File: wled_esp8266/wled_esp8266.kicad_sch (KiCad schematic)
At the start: 34 parts, among them J1 PWR, J2 Conn_01x05, J3 Screw_Terminal_01x04, J4 LED_STRIPT, J5 USB_B_Micro, Q1 IRF3708, Q2 IRF3708, Q3 IRF3708, U1 ESP-12F, U2 AMS1117-3.3

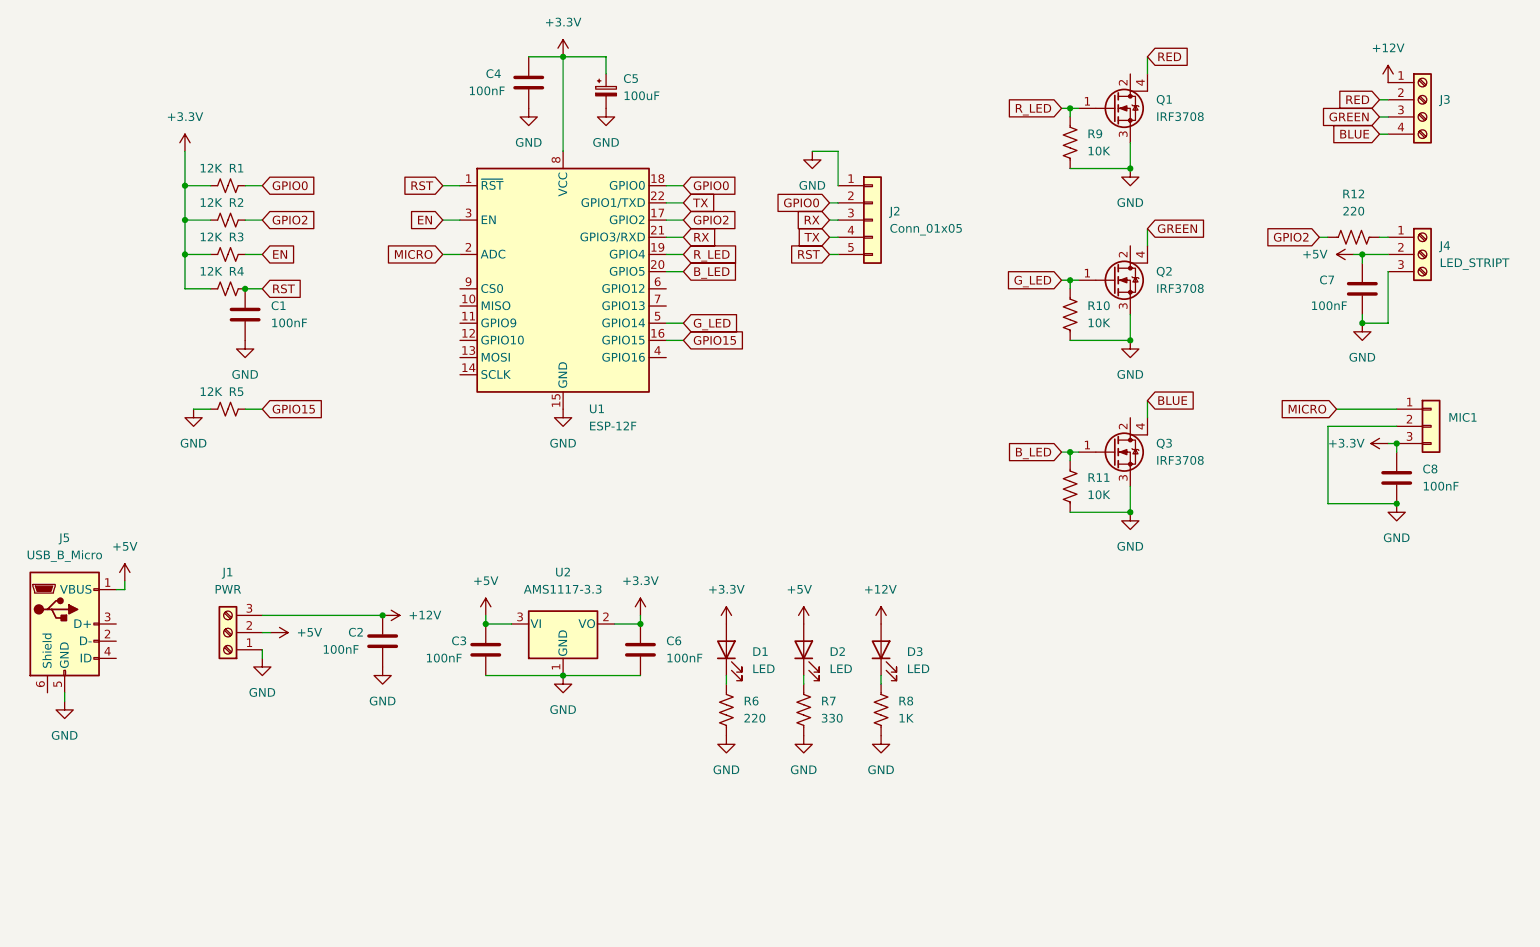
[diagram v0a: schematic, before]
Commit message: update new pcb
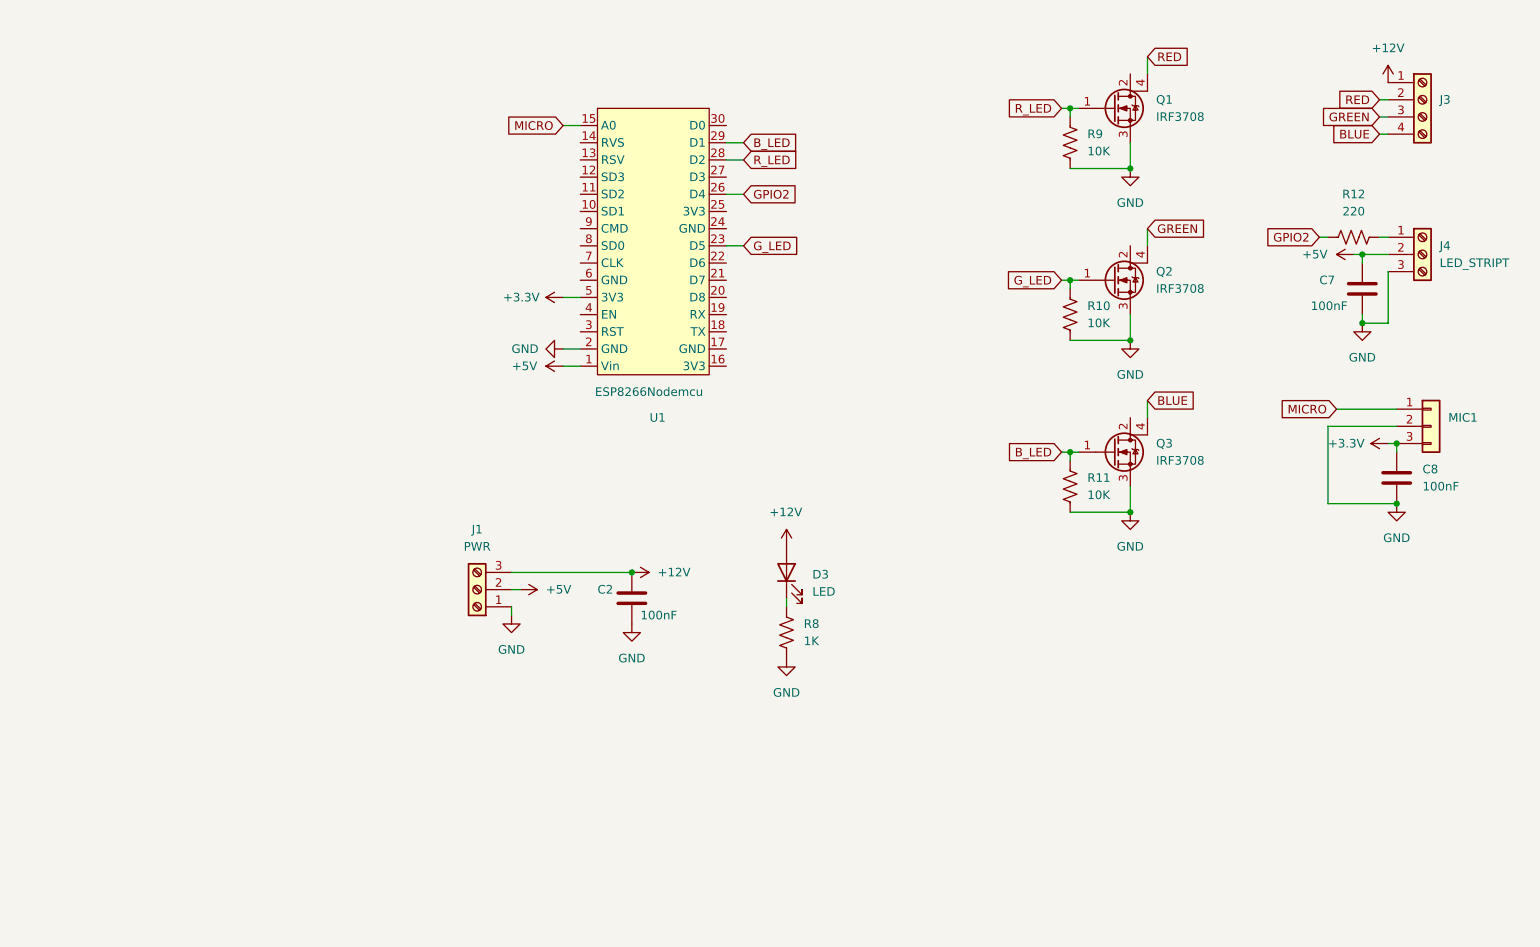
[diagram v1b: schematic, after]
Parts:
- removed C1, C3, C4, C6: 100nF, Capacitor_SMD:C_0805_2012Metric_Pad1.18x1.45mm_HandSolder, symbol Device:C
- removed C5: 100uF, Capacitor_Tantalum_SMD:CP_EIA-3528-12_Kemet-T_Pad1.50x2.35mm_HandSolder, symbol Device:C_Polarized_Small
- removed D1, D2: LED, LED_SMD:LED_0805_2012Metric_Pad1.15x1.40mm_HandSolder, symbol Device:LED
- removed J2: Conn_01x05, Connector_PinSocket_2.54mm:PinSocket_1x05_P2.54mm_Vertical, symbol Connector_Generic:Conn_01x05
- removed J5: USB_B_Micro, Connector_USB:USB_Micro, symbol Connector:USB_B_Micro
- removed R1, R2, R3, R4, R5: 12K, Resistor_SMD:R_0805_2012Metric_Pad1.20x1.40mm_HandSolder, symbol Device:R_Small_US
- removed R6: 220, Resistor_SMD:R_0805_2012Metric_Pad1.20x1.40mm_HandSolder, symbol Device:R_US
- removed R7: 330, Resistor_SMD:R_0805_2012Metric_Pad1.20x1.40mm_HandSolder, symbol Device:R_US
- removed U1: ESP-12F, RF_Module:ESP-12E, symbol RF_Module:ESP-12F
- removed U2: AMS1117-3.3, Package_TO_SOT_SMD:SOT-223-3_TabPin2, symbol Regulator_Linear:AMS1117-3.3
- added U1: ESP8266Nodemcu, Module:ESP8266Nodemcu, symbol MCU_Module:ESP8266Nodemcu
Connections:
- net +3V3: now also U1.5 (3V3)
- net +5V: now also U1.1 (Vin)
- net B_LED: now also U1.29 (D1)
- net GND: now also U1.2 (GND)
- net GPIO2: now also U1.26 (D4)
- net G_LED: now also U1.23 (D5)
- net MICRO: now also U1.15 (A0)
- net R_LED: now also U1.28 (D2)
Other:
- moved on the sheet: C2, D3, R8

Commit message: update PCB
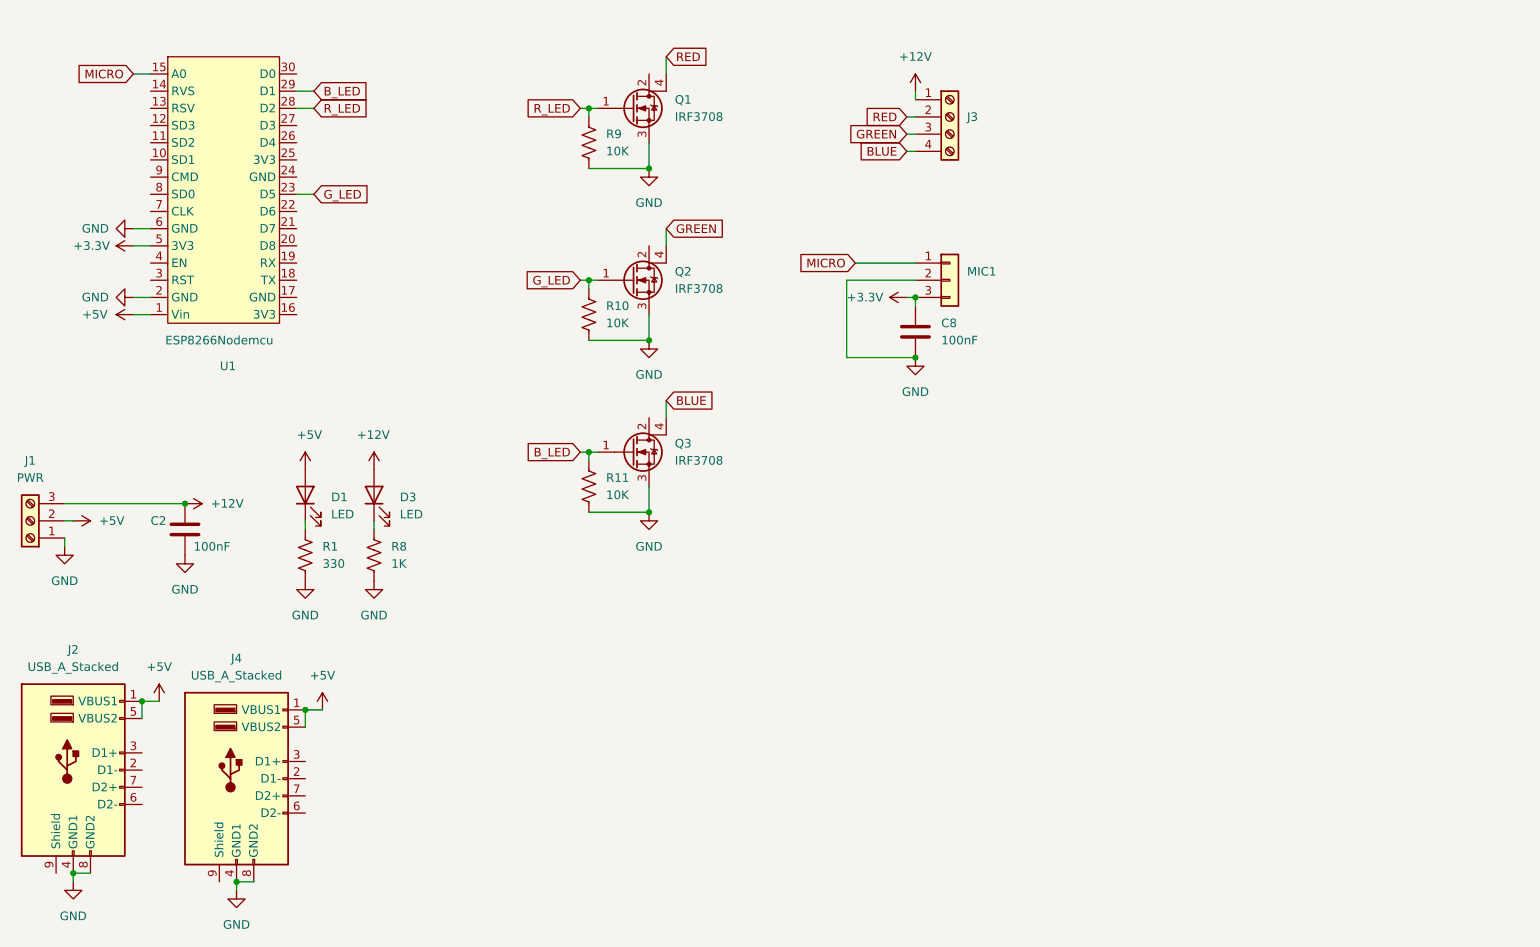
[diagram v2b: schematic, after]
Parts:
- removed C7: 100nF, Capacitor_SMD:C_0805_2012Metric_Pad1.18x1.45mm_HandSolder, symbol Device:C
- removed J4: LED_STRIPT, TerminalBlock:TerminalBlock_bornier-3_P5.08mm, symbol Connector:Screw_Terminal_01x03
- removed R12: 220, Resistor_SMD:R_0805_2012Metric_Pad1.20x1.40mm_HandSolder, symbol Device:R_US
- added D1: LED, LED_THT:LED_D3.0mm, symbol Device:LED
- added J2, J4: USB_A_Stacked, Connector_USB:USB_A_Wuerth_61400826021_Horizontal_Stacked, symbol Connector:USB_A_Stacked
- added R1: 330, Resistor_SMD:R_0805_2012Metric_Pad1.20x1.40mm_HandSolder, symbol Device:R_US
- D3: footprint LED_SMD:LED_0805_2012Metric_Pad1.15x1.40mm_HandSolder -> LED_THT:LED_D3.0mm
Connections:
- net +5V: now also D1.2 (A), J2.1 (VBUS1), J2.5 (VBUS2), J4.1 (VBUS1), J4.5 (VBUS2)
- net GND: now also U1.6 (GND), J2.4 (GND1), J2.8 (GND2), J4.4 (GND1), J4.8 (GND2), R1.2
- net GPIO2: no longer names the net of U1.26 (D4)
- new net: D1.1 (K), R1.1
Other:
- moved on the sheet: C2, C8, D3, J1, J3, MIC1, Q1, Q2, Q3, R10, R11, R8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

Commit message: update PCB
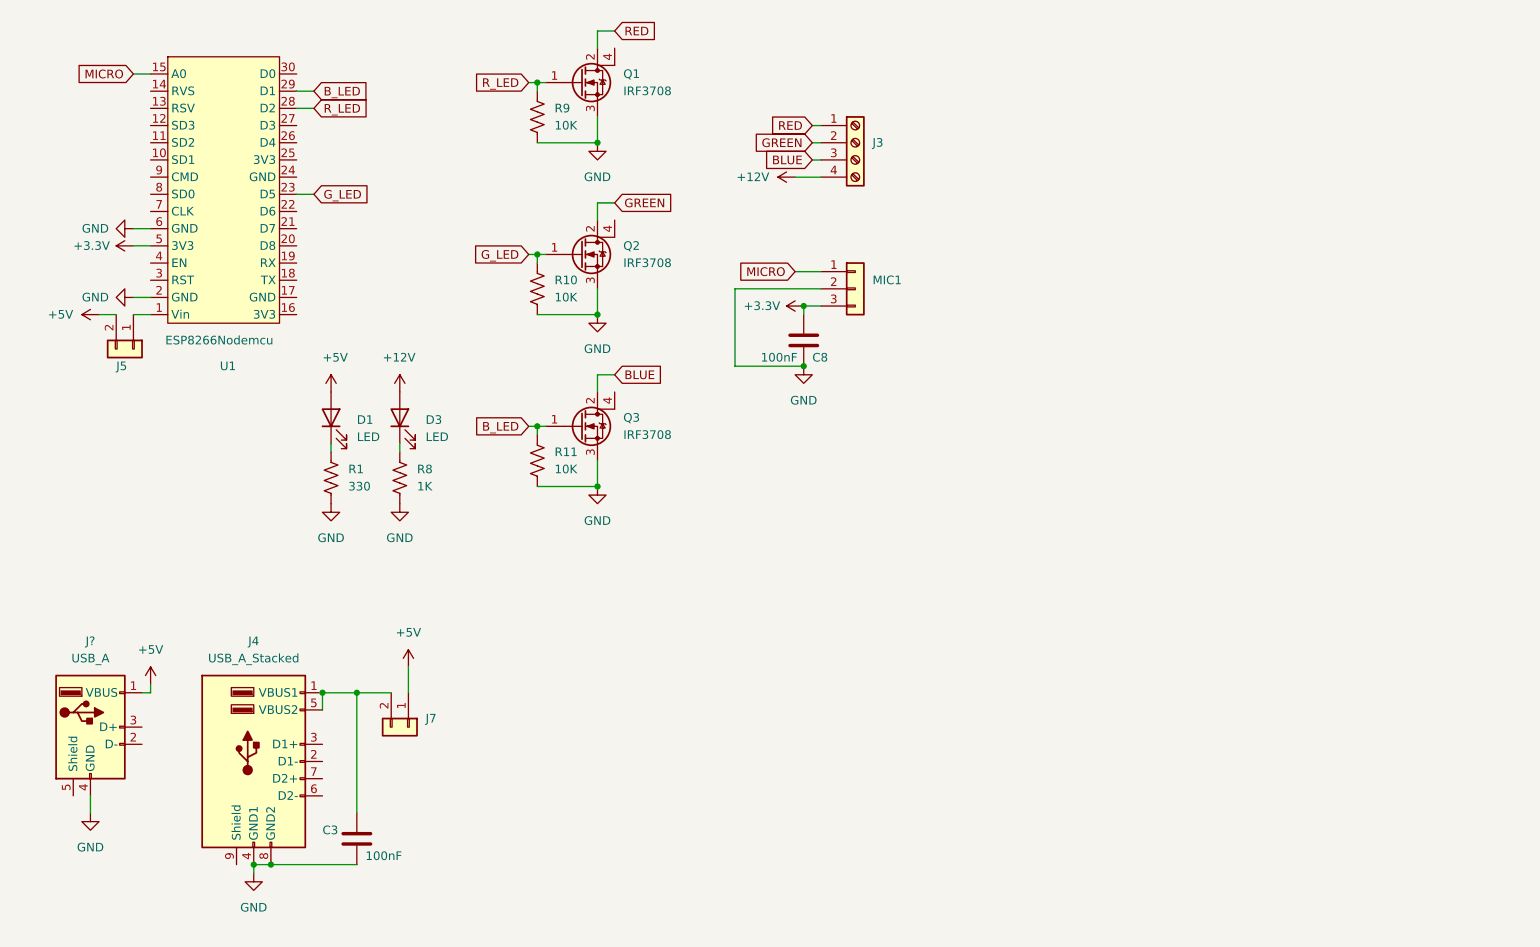
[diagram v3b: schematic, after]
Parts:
- removed C2: 100nF, Capacitor_SMD:C_0805_2012Metric_Pad1.18x1.45mm_HandSolder, symbol Device:C
- removed J1: PWR, TerminalBlock:TerminalBlock_bornier-3_P5.08mm, symbol Connector:Screw_Terminal_01x03
- removed J2: USB_A_Stacked, Connector_USB:USB_A_Wuerth_61400826021_Horizontal_Stacked, symbol Connector:USB_A_Stacked
- added C3: 100nF, Capacitor_SMD:C_0805_2012Metric_Pad1.18x1.45mm_HandSolder, symbol Device:C
- added J5, J7: Conn_01x02, Connector_PinSocket_2.54mm:PinSocket_1x02_P2.54mm_Vertical, symbol Connector_Generic:Conn_01x02
- added J?: USB_A, symbol Connector:USB_A
- Q1, Q2, Q3: footprint Package_TO_SOT_SMD:TO-252-3_TabPin4 -> Package_TO_SOT_SMD:TO-252-2
- U1: footprint Module:ESP8266Nodemcu -> Module:LoLinNodeMcu(esp8266)
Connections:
- net +12V: now also J3.4 (Pin_4); no longer J3.1 (Pin_1)
- net +5V: now also J5.2 (Pin_2), J7.1 (Pin_1), J?.1 (VBUS); no longer J4.1 (VBUS1), J4.5 (VBUS2), U1.1 (Vin)
- net BLUE: now also J3.3 (Pin_3), Q3.2 (D); no longer J3.4 (Pin_4), Q3.4 (D)
- net GND: now also C3.2, J?.4 (GND)
- net GREEN: now also J3.2 (Pin_2), Q2.2 (D); no longer J3.3 (Pin_3), Q2.4 (D)
- net RED: now also J3.1 (Pin_1), Q1.2 (D); no longer J3.2 (Pin_2), Q1.4 (D)
- new net: C3.1, J4.1 (VBUS1), J4.5 (VBUS2), J7.2 (Pin_2)
- new net: J5.1 (Pin_1), U1.1 (Vin)
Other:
- moved on the sheet: C8, D1, D3, J3, J4, MIC1, Q1, Q2, Q3, R1, R10, R11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
